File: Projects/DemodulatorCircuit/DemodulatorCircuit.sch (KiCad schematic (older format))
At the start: 22 parts, among them IC2 MC74ACT86DG, J1 SMA-J-P-H-ST-EM1, J2 Conn_01x02, J3 SMA-J-P-H-ST-EM1, U1 TLV3501AID, U2 TLV2374ID, U3 SFECF10M7EA00-R0, U4 SN74ACT04IDREP

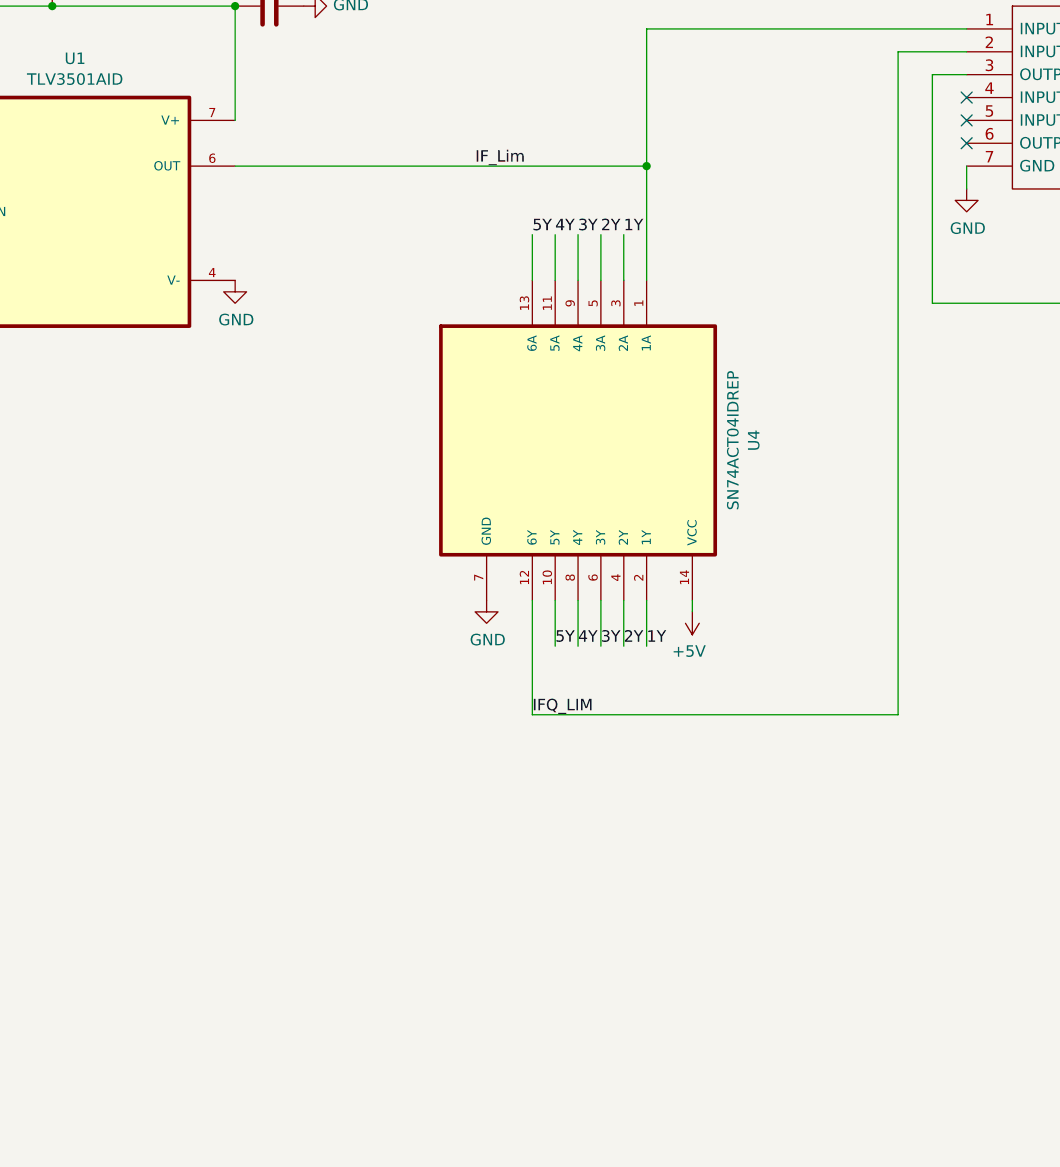
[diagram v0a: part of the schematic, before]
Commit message: This is the latest version with updated footprints etc
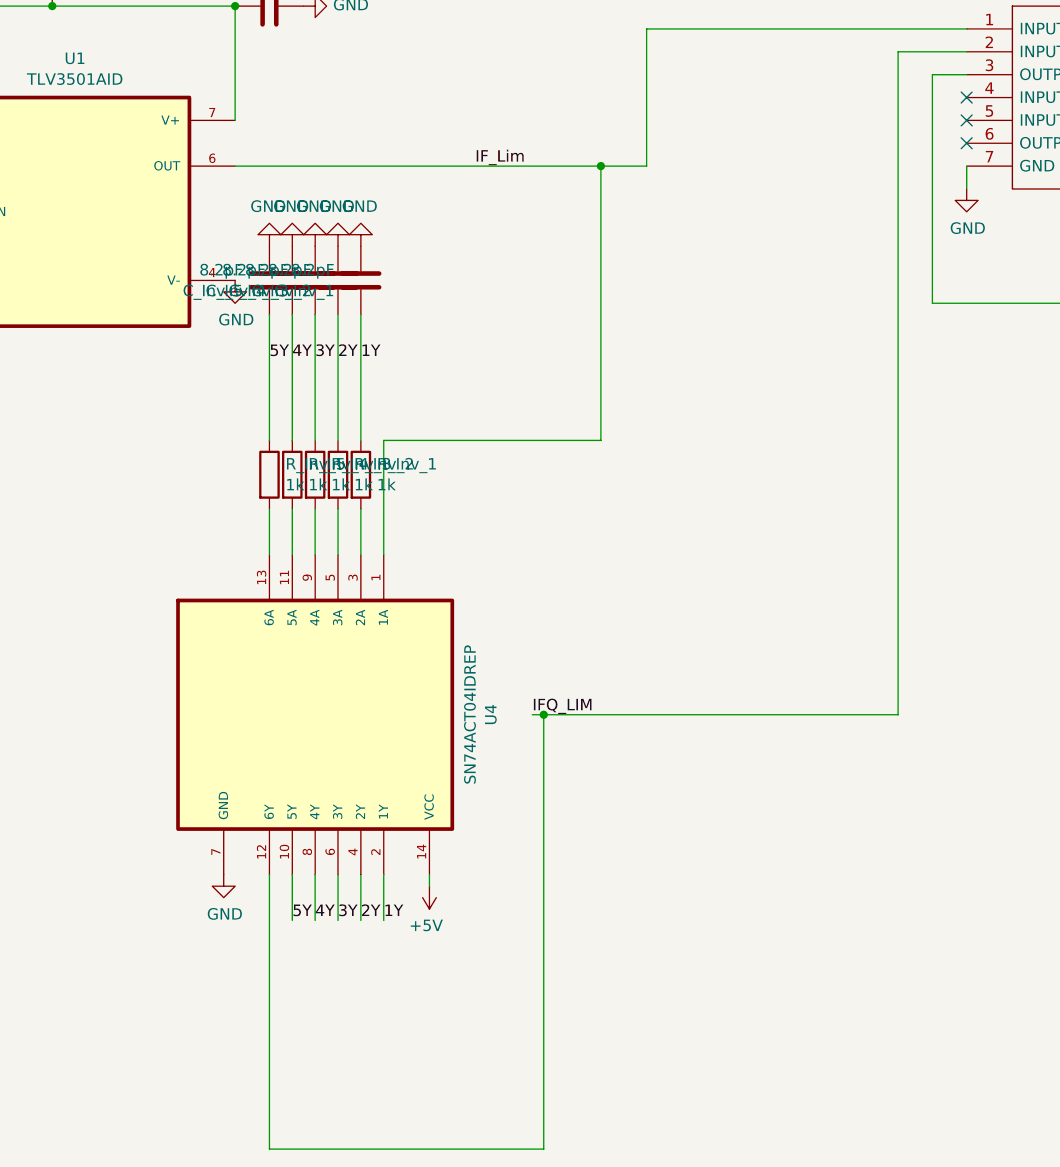
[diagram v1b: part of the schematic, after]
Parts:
- added C_Inv_1, C_Inv_2, C_Inv_3, C_Inv_4, C_Inv_5: 8.2pF, Capacitor_SMD:C_0603_1608Metric, symbol Device:C
- added R_Inv_1, R_Inv_2, R_Inv_3, R_Inv_4, R_Inv_5: 1k, Resistor_SMD:R_0603_1608Metric, symbol Device:R
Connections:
- net 1Y: now also C_Inv_1.1, R_Inv_1.1; no longer U4.3 (2A)
- net 2Y: now also C_Inv_2.1, R_Inv_2.1; no longer U4.5 (3A)
- net 3Y: now also C_Inv_3.1, R_Inv_3.1; no longer U4.9 (4A)
- net 4Y: now also C_Inv_4.1, R_Inv_4.1; no longer U4.11 (5A)
- net 5Y: now also C_Inv_5.1, R_Inv_5.1; no longer U4.13 (6A)
- net GND: now also C_Inv_1.2, C_Inv_2.2, C_Inv_3.2, C_Inv_4.2, C_Inv_5.2
- new net: R_Inv_1.2, U4.3 (2A)
- new net: R_Inv_2.2, U4.5 (3A)
- new net: R_Inv_3.2, U4.9 (4A)
- new net: R_Inv_4.2, U4.11 (5A)
- new net: R_Inv_5.2, U4.13 (6A)
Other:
- moved on the sheet: U4
